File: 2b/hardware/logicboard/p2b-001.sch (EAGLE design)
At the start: 72 parts, among them IC1 74LS06N, IC2 4066N, J1 MKR, J10 1-Wire, J2 GPIO, J20 GPIO, J3 Vcc, J4** RLY2, J5 SPI, J6 LED, J7 DIN5, J8 DIN5, J9 DIN5, K1 G5V1, Q1 220mA/50V/3.5Ω, Q2 220mA/50V/3.5Ω, T1 2SC1815

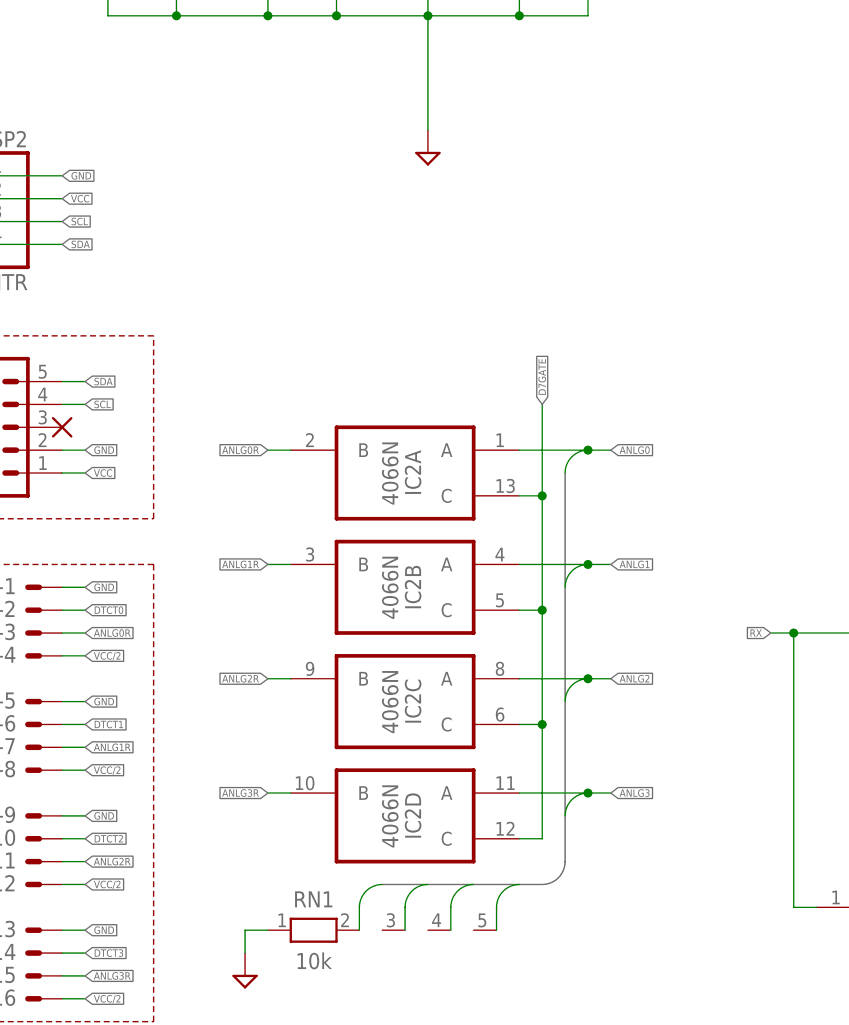
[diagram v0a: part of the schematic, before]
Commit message: Fixed P2b.
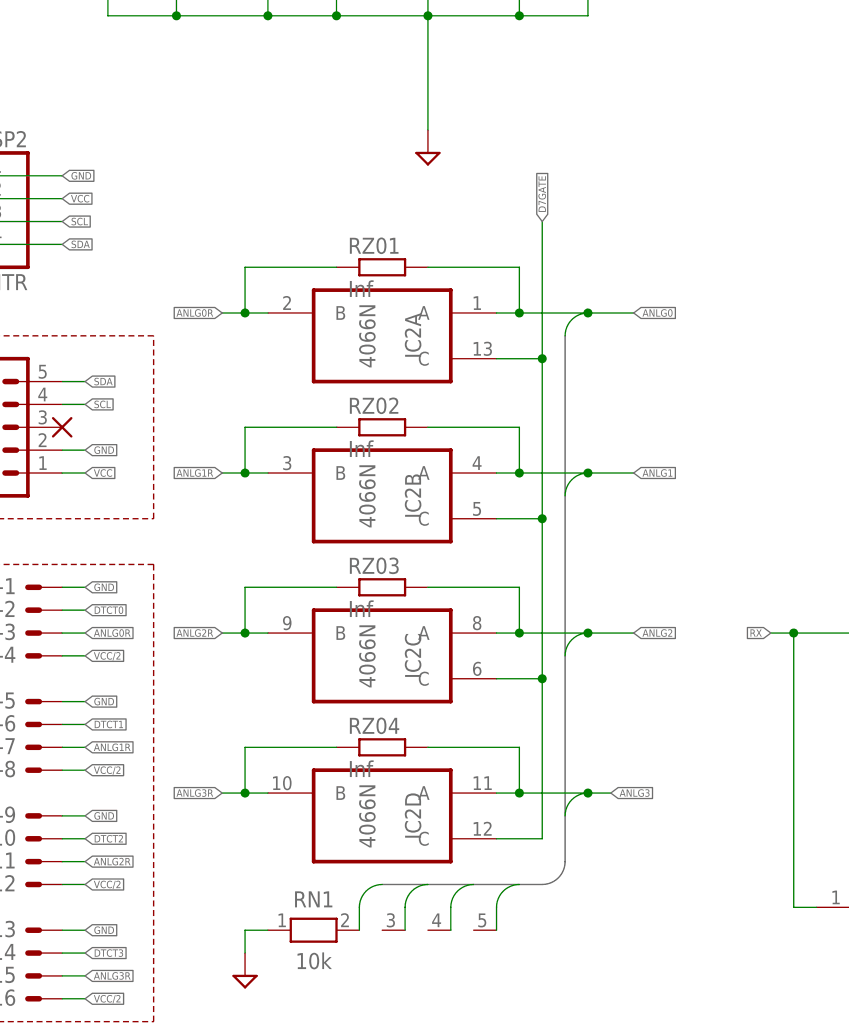
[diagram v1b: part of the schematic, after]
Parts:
- added RZ01, RZ02, RZ03, RZ04: Inf, rcl:R-EU_M2012
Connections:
- net ANLG0: now also RZ01.2
- net ANLG0R: now also RZ01.1
- net ANLG1: now also RZ02.2
- net ANLG1R: now also RZ02.1
- net ANLG2: now also RZ03.2
- net ANLG2R: now also RZ03.1
- net ANLG3: now also RZ04.2
- net ANLG3R: now also RZ04.1
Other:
- moved on the sheet: IC2A, IC2B, IC2C, IC2D
